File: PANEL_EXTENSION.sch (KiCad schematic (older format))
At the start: 24 parts, among them J5 Conn_01x08_Male, U20 SGM3157YC6, U21 SGM3157YC6, U22 CM1293A-04SO, U23 CM1293A-04SO, U24 CM1293A-04SO

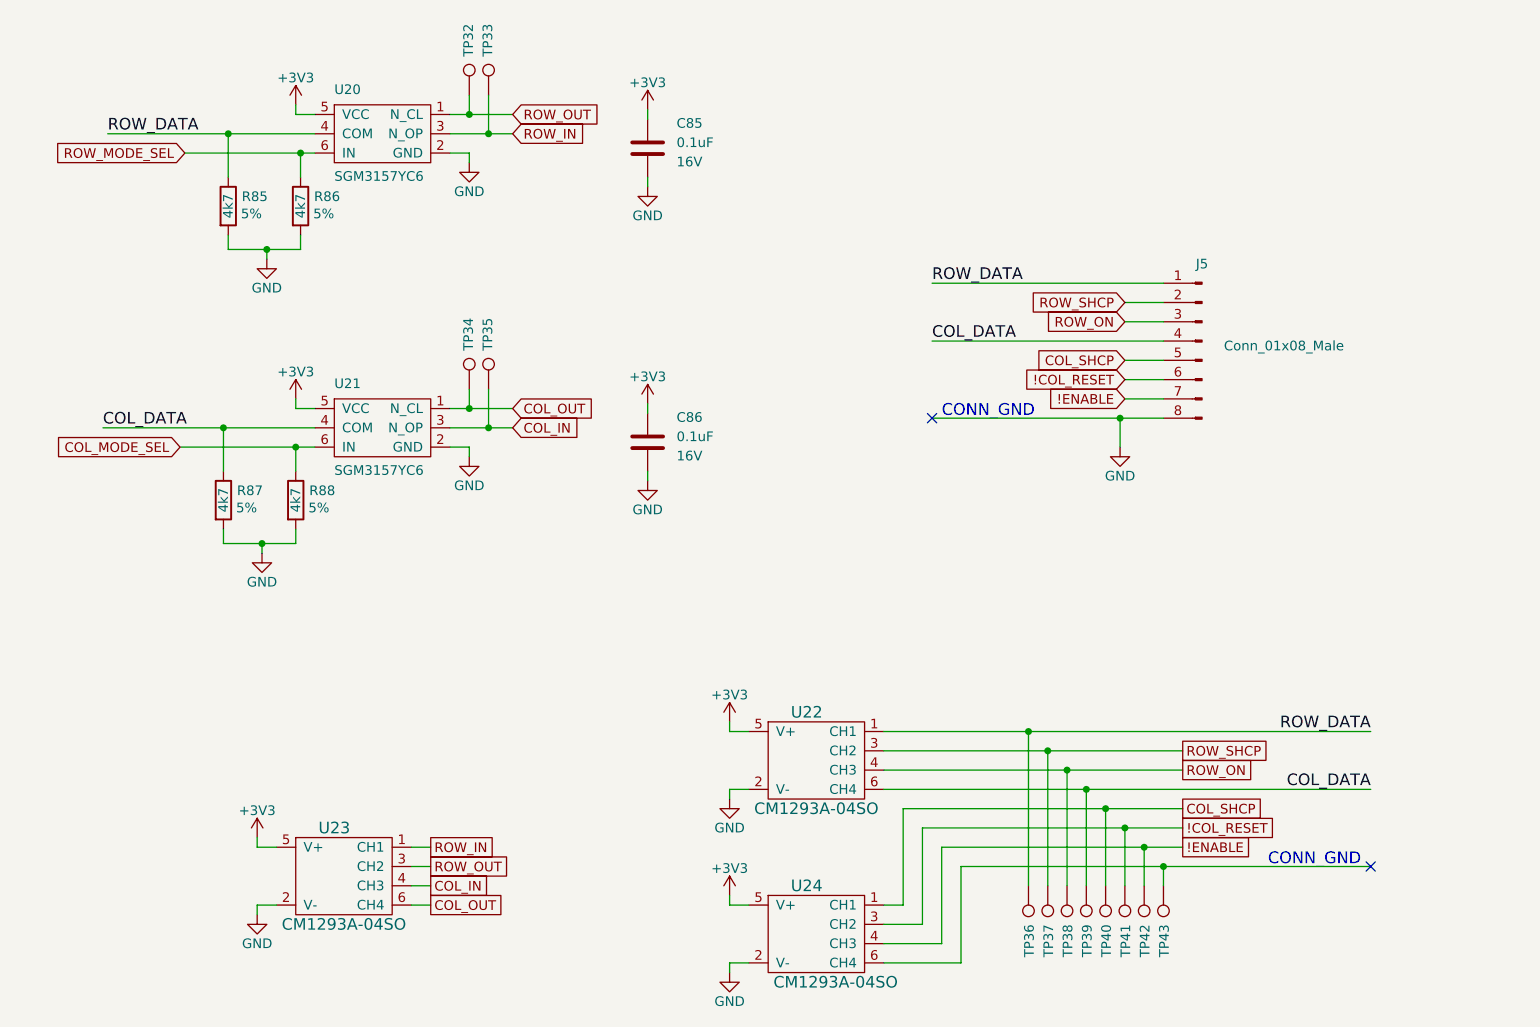
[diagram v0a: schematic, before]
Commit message: automated commit
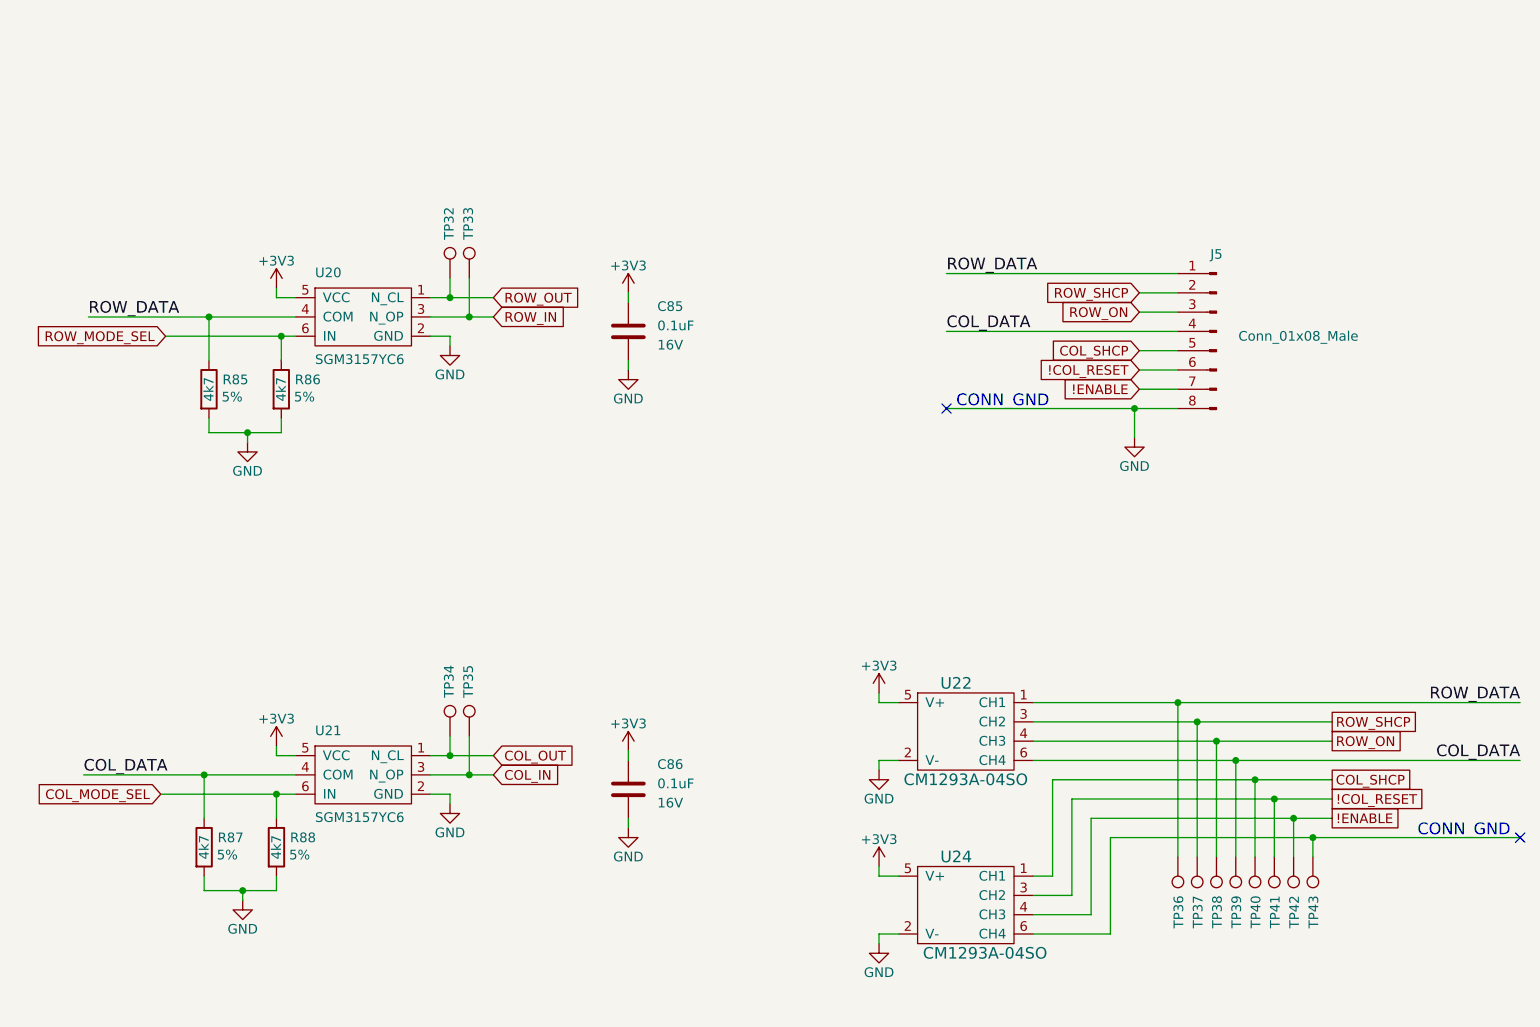
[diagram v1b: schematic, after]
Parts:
- removed U23: CM1293A-04SO, symbol custom:CM1293A-04SO_ALTERNATE_SYMBOL
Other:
- moved on the sheet: C85, C86, J5, R85, R86, R87, R88, TP32, TP33, TP34, TP35, TP36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
